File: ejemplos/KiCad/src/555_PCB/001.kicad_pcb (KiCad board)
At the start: 2 copper layers, 37.2 x 73.4 mm, 13 parts, among them J1 CONN_01X04

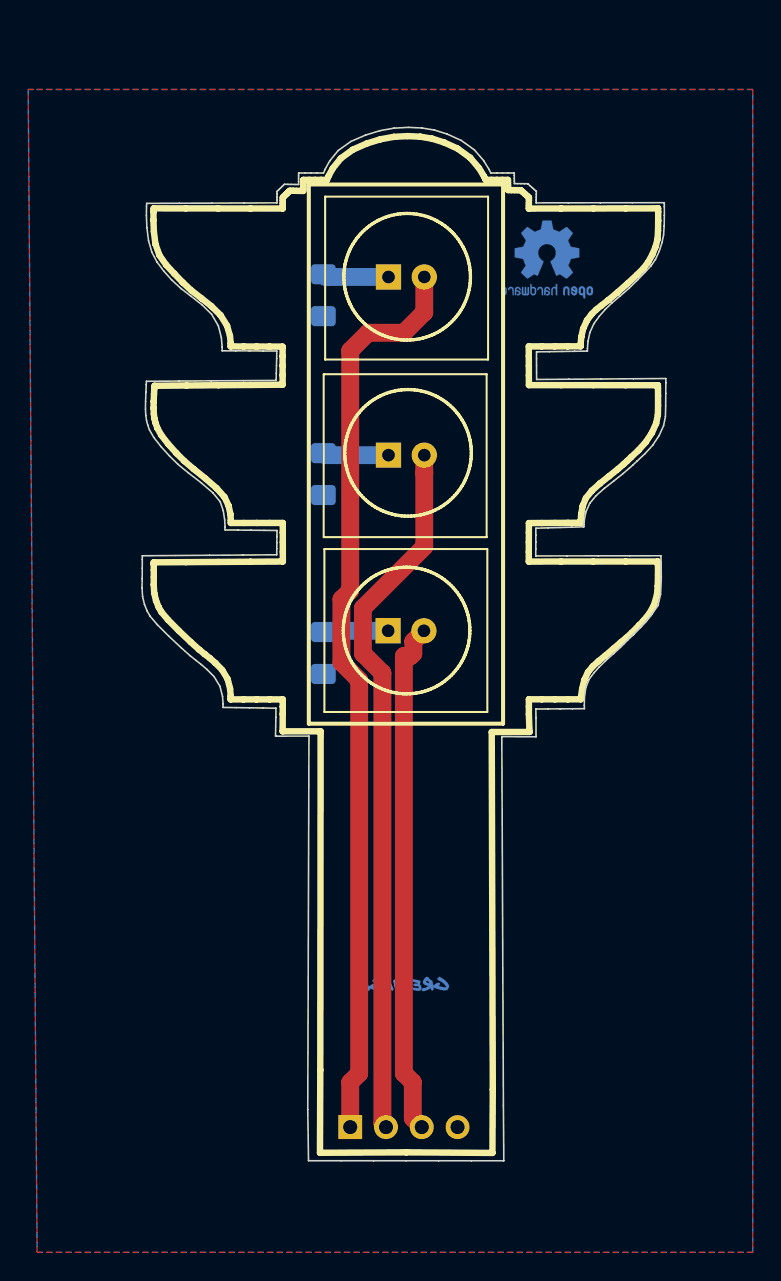
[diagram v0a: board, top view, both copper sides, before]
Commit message: Auto stash before merge of "master" and "origin/master"
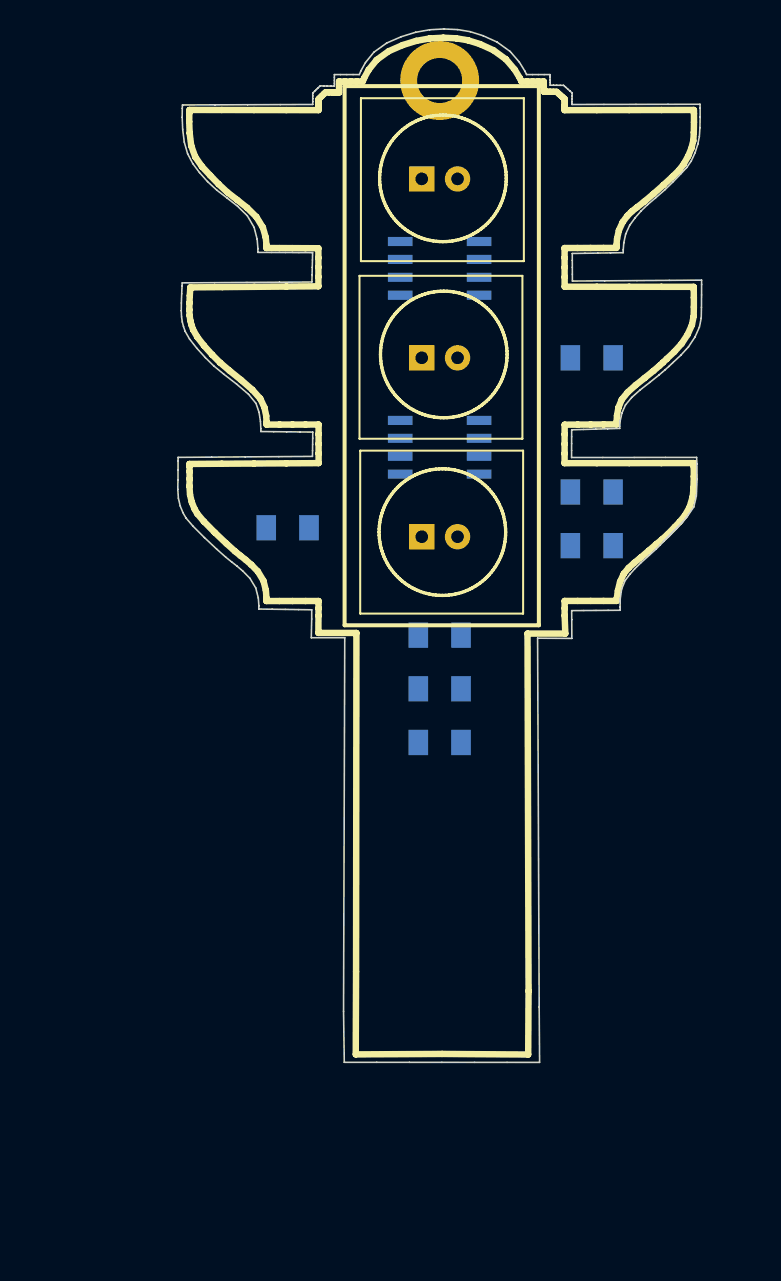
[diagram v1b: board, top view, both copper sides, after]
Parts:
- removed J1: CONN_01X04, Semaforo:PinHeader_1x04_P2.54mm_Vertical
- removed the REF** at (134.0, 118.1)
- removed the REF** at (144.1, 81.9) (x2)
- removed svg2mod: G***, MazBot-Botonera-02:Developed-Silks3
- removed svg2mod: G***, MazBot-Botonera-02:GReynaga.CuMask3
- added C1: 100uF, Capacitor_SMD:C_1206_3216Metric_Pad1.39x1.80mm_HandSolder, B.Cu at (136.5, 108.6)
- added C2: C, Capacitor_SMD:C_1206_3216Metric_Pad1.39x1.80mm_HandSolder, B.Cu at (136.5, 112.4)
- added R4: 470, Resistor_SMD:R_1206_3216Metric_Pad1.39x1.80mm_HandSolder, B.Cu at (147.3, 98.4)
- added R5: 47k, Resistor_SMD:R_1206_3216Metric_Pad1.39x1.80mm_HandSolder, B.Cu at (136.5, 116.2)
- added REF**: MountingHole_3.2mm_M3_DIN965_Pad, OshPark_Version:MountingHole_3.2mm_M3_DIN965_Pad, F.Cu at (136.5, 69.2)
- added U1: NE555, Wickerlib:SOIC-8-3.9x4.9MM-P1.27MM, B.Cu at (136.5, 82.5)
- added U2: NE555, Wickerlib:SOIC-8-3.9x4.9MM-P1.27MM, B.Cu at (136.5, 95.2)
- R1: value 330 -> 100k; footprint Resistor_SMD:R_1206_3216Metric_Pad1.42x1.75mm_HandSolder -> Resistor_SMD:R_1206_3216Metric_Pad1.39x1.80mm_HandSolder
- R2: value 330 -> 470; footprint Resistor_SMD:R_1206_3216Metric_Pad1.42x1.75mm_HandSolder -> Resistor_SMD:R_1206_3216Metric_Pad1.39x1.80mm_HandSolder
- R3: value 330 -> 220; footprint Resistor_SMD:R_1206_3216Metric_Pad1.42x1.75mm_HandSolder -> Resistor_SMD:R_1206_3216Metric_Pad1.39x1.80mm_HandSolder
- moved R3 28.3 mm to (147.3, 88.9), turned to 0 degrees
- moved R1 26.1 mm to (147.3, 102.2), turned to 0 degrees
- moved E1 7.43 mm to (136.5, 102.2)
- moved D1 7.35 mm to (135.3, 76.2)
- moved D2 7.30 mm to (135.3, 88.9)
- moved D3 7.09 mm to (135.3, 101.6)
- moved R2 4.58 mm to (125.7, 101.0), turned to 0 degrees
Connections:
- D3 pad 1: Net-(D3-Pad1) -> GND
- R1 pad 2: GND -> Net-(C1-Pad2)
- R2 pad 1: Net-(D2-Pad1) -> Net-(D1-Pad2)
- R2 pad 2: GND -> +12V
- R3 pad 1: Net-(D3-Pad1) -> +12V
- R3 pad 2: GND -> Net-(D2-Pad2)
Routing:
- net Net-(D1-Pad2): track 65.1 -> 0.00 mm
- net Net-(D2-Pad2): track 50.2 -> 0.00 mm
- net Net-(D3-Pad2): track 36.6 -> 0.00 mm
- net Net-(D1-Pad1): track 4.70 -> 0.00 mm
- net Net-(D2-Pad1): track 4.68 -> 0.00 mm
- net Net-(D3-Pad1): track 4.63 -> 0.00 mm
- removed copper zone on B.Cu, net GND
- removed copper zone on F.Cu, net GND
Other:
- board text removed: "10mm"
- board text removed: "GND"
- board text removed: "GREEN"
- board text removed: "RED"
- board text removed: "Traffic Light"
- board text removed: "YELLOW"
- board text removed: "v1.0"
